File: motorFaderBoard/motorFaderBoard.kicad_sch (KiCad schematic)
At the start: 18 parts, among them J1 Conn_01x08_Pin, J2 Conn_01x08_Socket, U1 ADS1115IDGS, U2 PCF8574T, U3 L293DD

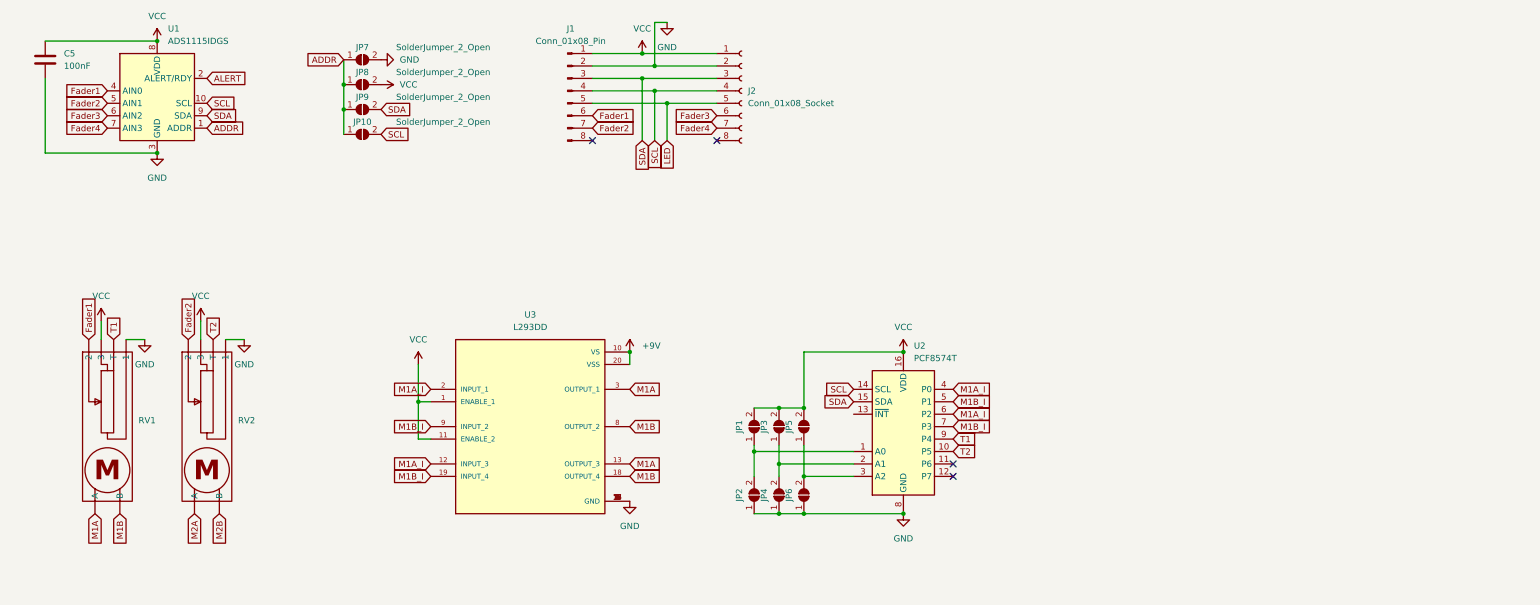
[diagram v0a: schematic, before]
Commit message: pcb and stuff
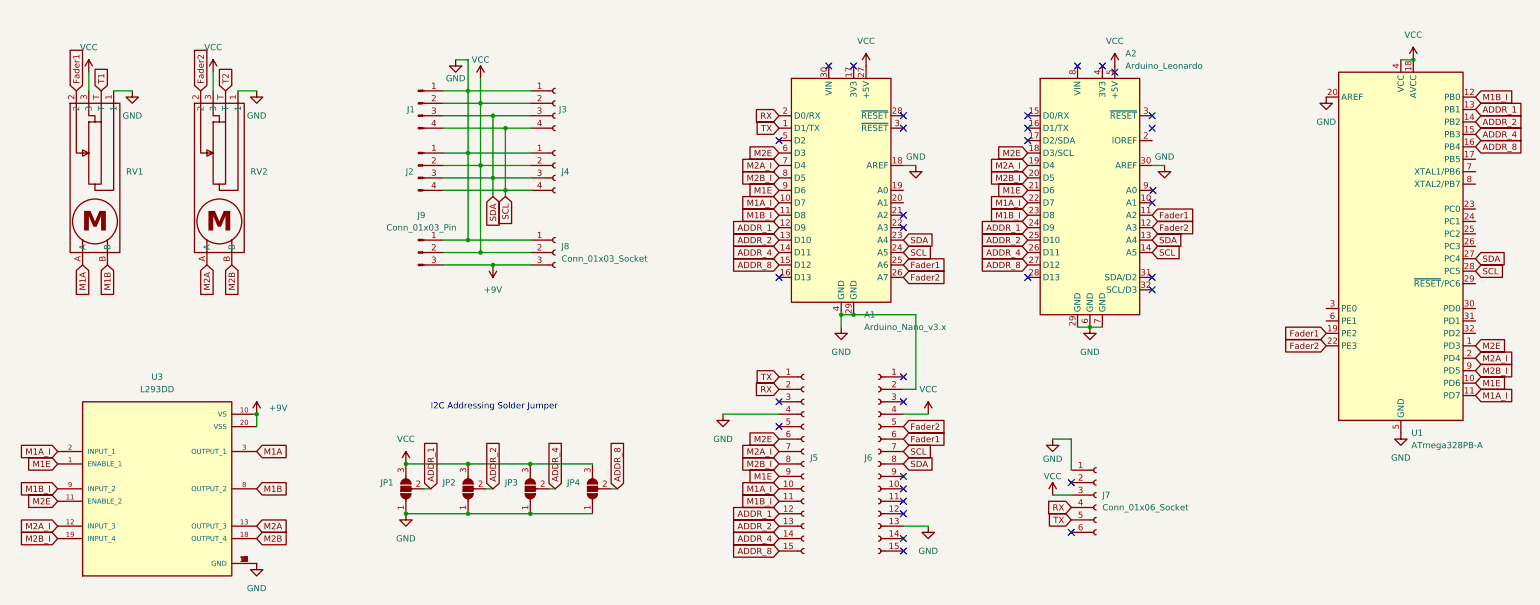
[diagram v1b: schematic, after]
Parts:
- removed C5: 100nF, Capacitor_SMD:C_0805_2012Metric_Pad1.18x1.45mm_HandSolder, symbol Device:C
- removed J1: Conn_01x08_Pin, symbol Connector:Conn_01x08_Pin
- removed J2: Conn_01x08_Socket, symbol Connector:Conn_01x08_Socket
- removed JP1, JP10, JP2, JP3, JP4, JP5, JP6, JP7, JP8, JP9: SolderJumper_2_Open, Jumper:SolderJumper-2_P1.3mm_Open_RoundedPad1.0x1.5mm, symbol Jumper:SolderJumper_2_Open
- removed U1: ADS1115IDGS, Package_SO:TSSOP-10_3x3mm_P0.5mm, symbol Analog_ADC:ADS1115IDGS
- removed U2: PCF8574T, Package_SO:SOIC-16W_7.5x10.3mm_P1.27mm, symbol Interface_Expansion:PCF8574T
- added A1: Arduino_Nano_v3.x, Module:Arduino_Nano, symbol MCU_Module:Arduino_Nano_v3.x
- added A2: Arduino_Leonardo, Module:Arduino_UNO_R3, symbol MCU_Module:Arduino_Leonardo
- added J1, J2: Conn_01x04_Pin, Connector_PinHeader_2.54mm:PinHeader_1x04_P2.54mm_Vertical, symbol Connector:Conn_01x04_Pin
- added J3, J4: Conn_01x04_Socket, Connector_PinSocket_2.54mm:PinSocket_1x04_P2.54mm_Vertical, symbol Connector:Conn_01x04_Socket
- added J5, J6: Conn_01x15_Socket, Connector_PinSocket_2.54mm:PinSocket_1x15_P2.54mm_Vertical_SMD_Pin1Right, symbol Connector:Conn_01x15_Socket
- added J7: Conn_01x06_Socket, Connector_PinSocket_2.54mm:PinSocket_1x05_P2.54mm_Vertical, symbol Connector:Conn_01x06_Socket
- added J8: Conn_01x03_Socket, Connector_PinSocket_2.54mm:PinSocket_1x03_P2.54mm_Vertical, symbol Connector:Conn_01x03_Socket
- added J9: Conn_01x03_Pin, Connector_PinHeader_2.54mm:PinHeader_1x03_P2.54mm_Vertical, symbol Connector:Conn_01x03_Pin
- added JP1, JP2, JP3, JP4: SolderJumper_3_Open, Jumper:SolderJumper-3_P2.0mm_Open_TrianglePad1.0x1.5mm, symbol Jumper:SolderJumper_3_Open
- added U1: ATmega328PB-A, Package_QFP:TQFP-32_7x7mm_P0.8mm, symbol MCU_Microchip_ATmega:ATmega328PB-A
- RV1, RV2: footprint (none) -> MotorFader:RES-TH_L146.5-W18.0_RSA0N11M9A07
- U3: footprint L293DD:SOIC127P1032X265-20N -> Package_SO:Infineon_SOIC-20W_7.6x12.8mm_P1.27mm
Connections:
- net +9V: now also J8.3 (Pin_3), J9.3 (Pin_3)
- net Fader1: now also RV1.2, A1.25 (A6), A2.11 (A2), J6.6 (Pin_6), U1.19 (PE2); no longer RV1. (1)
- net Fader2: now also RV2.2, A1.26 (A7), A2.12 (A3), J6.5 (Pin_5), U1.22 (PE3); no longer RV2. (1)
- net GND: now also RV1.1, RV2.1, A1.18 (AREF), A1.29 (GND), A1.4 (GND), A2.29 (GND), A2.30 (AREF), A2.6 (GND), A2.7 (GND), J1.1 (Pin_1), J2.1 (Pin_1), J3.1 (Pin_1), J4.1 (Pin_1), J5.4 (Pin_4), J6.13 (Pin_13), J6.2 (Pin_2), J7.1 (Pin_1), J8.1 (Pin_1), J9.1 (Pin_1), JP1.1 (A), JP2.1 (A), JP3.1 (A), JP4.1 (A), U1.20 (AREF), U1.21 (GND), U1.5 (GND); no longer RV1. (1), RV2. (1)
- net M1A: now also RV1.A; no longer RV1. (1), U3.13 (OUTPUT_3)
- net M1A_I: now also A1.10 (D7), A2.22 (D7), J5.10 (Pin_10), U1.11 (PD7); no longer U3.12 (INPUT_3)
- net M1B: now also RV1.B; no longer RV1. (1), U3.18 (OUTPUT_4)
- net M1B_I: now also A1.11 (D8), A2.23 (D8), J5.11 (Pin_11), U1.12 (PB0); no longer U3.19 (INPUT_4)
- net M2A: now also RV2.A, U3.13 (OUTPUT_3); no longer RV2. (1)
- net M2B: now also RV2.B, U3.18 (OUTPUT_4); no longer RV2. (1)
- net SCL: now also A1.24 (A5), A2.14 (A5), J1.4 (Pin_4), J2.4 (Pin_4), J3.4 (Pin_4), J4.4 (Pin_4), J6.7 (Pin_7), U1.28 (PC5)
- net SDA: now also A1.23 (A4), A2.13 (A4), J1.3 (Pin_3), J2.3 (Pin_3), J3.3 (Pin_3), J4.3 (Pin_3), J6.8 (Pin_8), U1.27 (PC4)
- net T1: now also RV1.T; no longer RV1. (1)
- net T2: now also RV2.T; no longer RV2. (1)
- net VCC: now also RV1.3, RV2.3, A1.27 (+5V), A2.5 (+5V), J1.2 (Pin_2), J2.2 (Pin_2), J3.2 (Pin_2), J4.2 (Pin_2), J6.4 (Pin_4), J7.3 (Pin_3), J8.2 (Pin_2), J9.2 (Pin_2), JP1.3 (B), JP2.3 (B), JP3.3 (B), JP4.3 (B), U1.18 (AVCC), U1.4 (VCC); no longer RV1. (1), RV2. (1), U3.1 (ENABLE_1), U3.11 (ENABLE_2)
- new net ADDR_1: A1.12 (D9), A2.24 (D9), J5.12 (Pin_12), JP1.2 (C), U1.13 (PB1)
- new net ADDR_2: A1.13 (D10), A2.25 (D10), J5.13 (Pin_13), JP2.2 (C), U1.14 (PB2)
- new net ADDR_4: A1.14 (D11), A2.26 (D11), J5.14 (Pin_14), JP3.2 (C), U1.15 (PB3)
- new net ADDR_8: A1.15 (D12), A2.27 (D12), J5.15 (Pin_15), JP4.2 (C), U1.16 (PB4)
- new net M1E: A1.9 (D6), A2.21 (D6), J5.9 (Pin_9), U1.10 (PD6), U3.1 (ENABLE_1)
- new net M2A_I: A1.7 (D4), A2.19 (D4), J5.7 (Pin_7), U1.2 (PD4), U3.12 (INPUT_3)
- new net M2B_I: A1.8 (D5), A2.20 (D5), J5.8 (Pin_8), U1.9 (PD5), U3.19 (INPUT_4)
- new net M2E: A1.6 (D3), A2.18 (D3/SCL), J5.6 (Pin_6), U1.1 (PD3), U3.11 (ENABLE_2)
- new net RX: A1.2 (D0/RX), J5.2 (Pin_2), J7.4 (Pin_4)
- new net TX: A1.1 (D1/TX), J5.1 (Pin_1), J7.5 (Pin_5)
- no-connect marks 4 -> 33
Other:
- note added: "I2C Addressing Solder Jumper"
- moved on the sheet: U3
